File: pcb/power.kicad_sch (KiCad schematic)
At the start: 17 parts

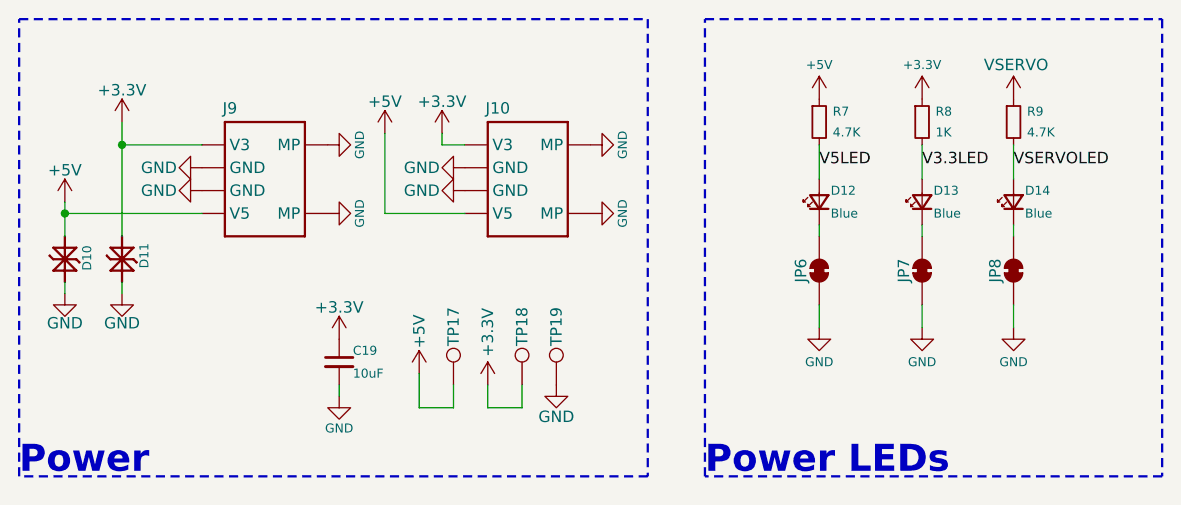
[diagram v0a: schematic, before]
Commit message: Updated symbols
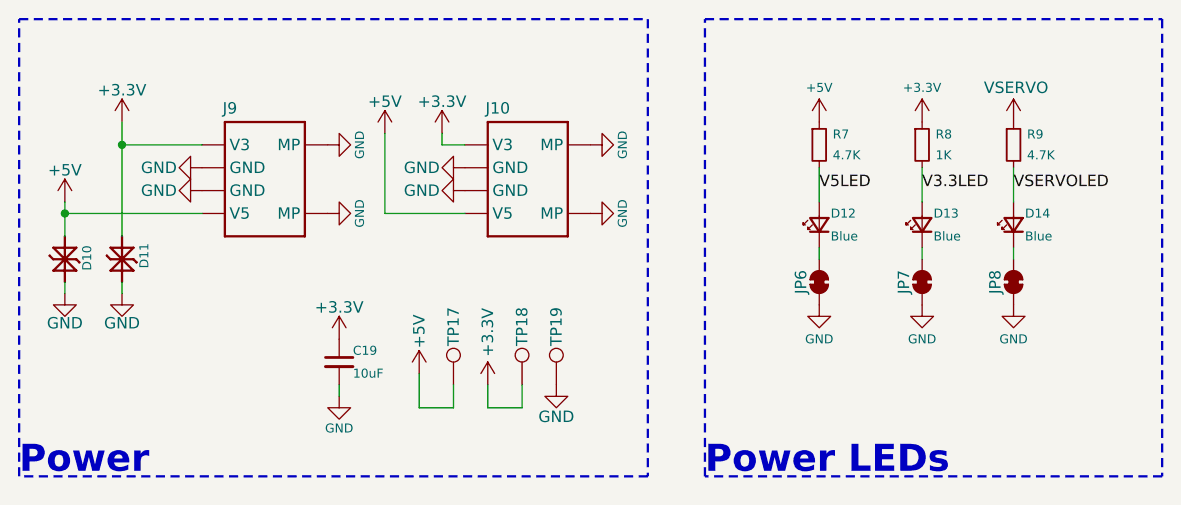
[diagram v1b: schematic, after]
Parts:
- JP6, JP7, JP8: value (none) -> SolderJumper_2_Bridged; footprint CRGM Connector:SolderJumper-2_P1.3mm_Bridged_RoundedPad1.0x1.5mm -> (none)
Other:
- moved on the sheet: D12, D13, D14, JP6, JP7, JP8, R7, R8, R9
